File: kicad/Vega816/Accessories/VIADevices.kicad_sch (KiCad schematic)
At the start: 13 parts, among them J102 VIA Port, U125 RC1602A

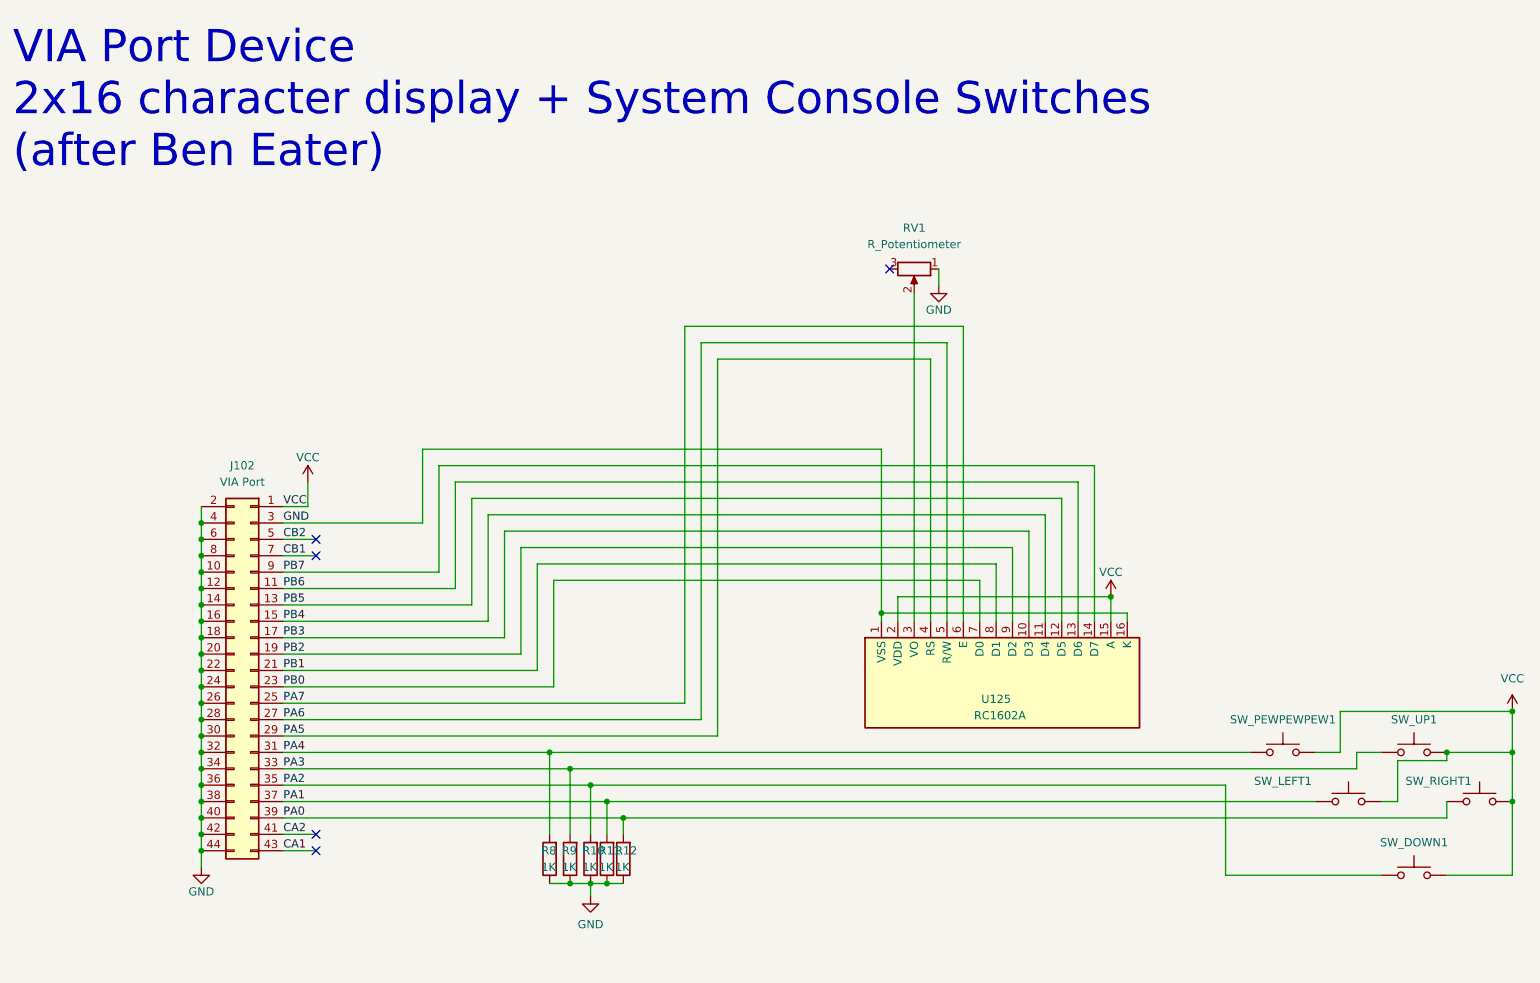
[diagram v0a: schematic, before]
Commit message: via
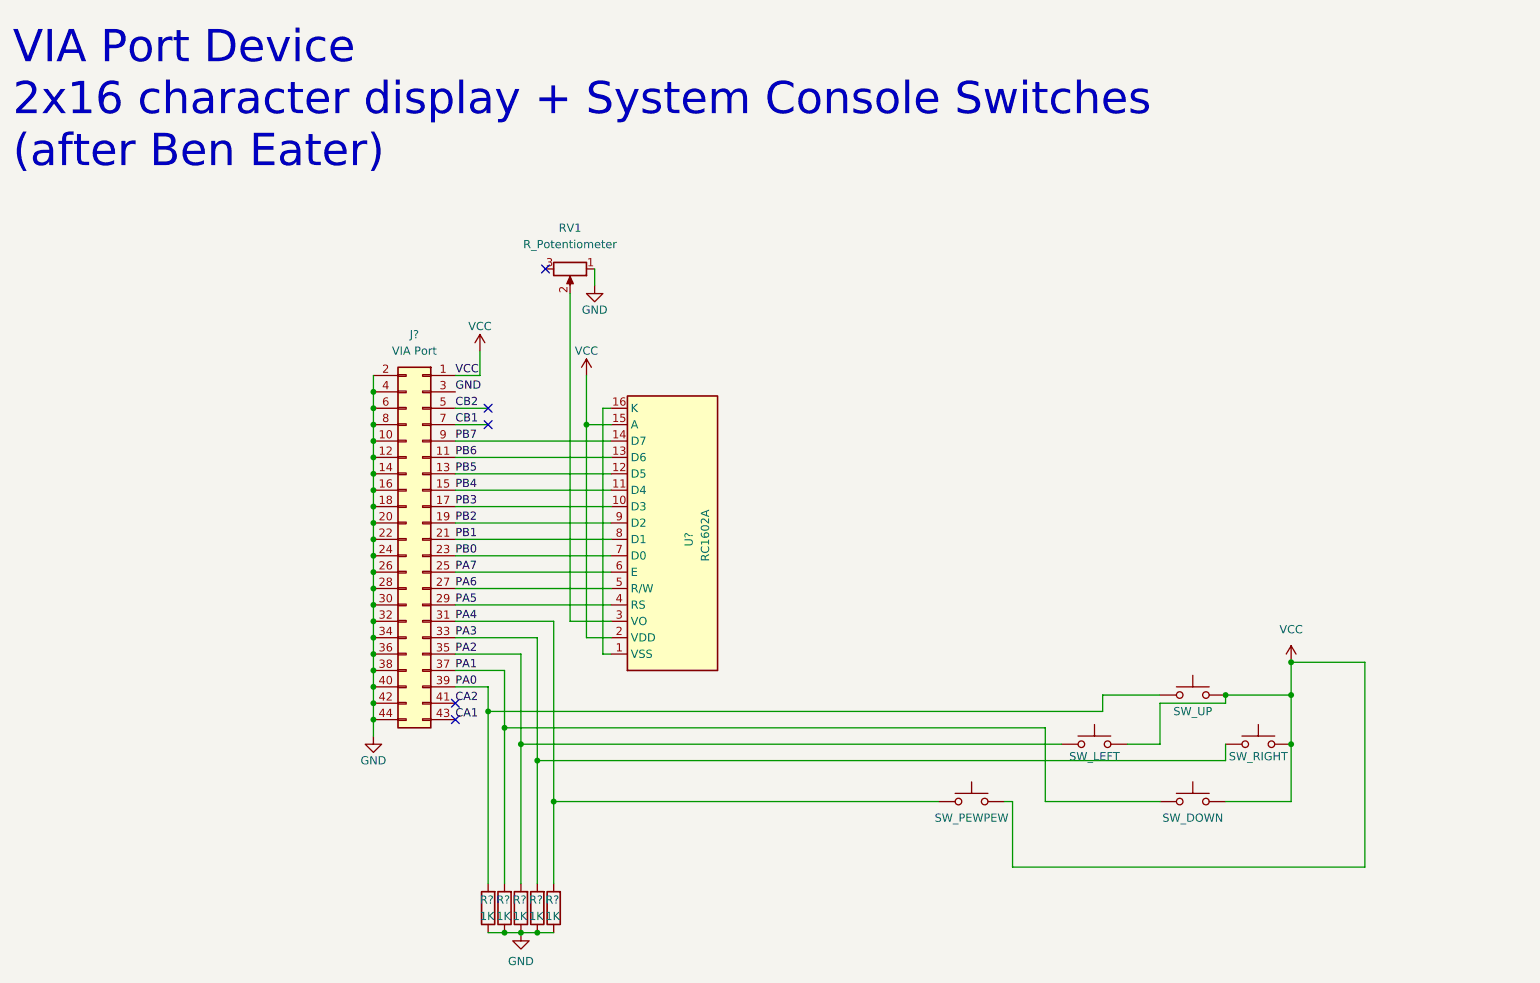
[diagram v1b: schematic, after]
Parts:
- removed J102: VIA Port, symbol Connector_Generic:Conn_02x22_Odd_Even
- removed R10, R11, R12, R8, R9: 1K, symbol Device:R
- removed SW_DOWN1, SW_LEFT1, SW_PEWPEWPEW1, SW_RIGHT1, SW_UP1: SW_Push, symbol Switch:SW_Push
- removed U125: RC1602A, Display:RC1602A, symbol Vega816:RC1602A
- added J?: VIA Port, symbol Connector_Generic:Conn_02x22_Odd_Even
- added R? (x5): 1K, symbol Device:R
- added SW_DOWN, SW_LEFT, SW_PEWPEW, SW_RIGHT, SW_UP: SW_Push, symbol Switch:SW_Push
- added U?: RC1602A, Display:RC1602A, symbol Vega816:RC1602A
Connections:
- net CA1: now also J?.43 (Pin_43)
- net CA2: now also J?.41 (Pin_41)
- net CB1: now also J?.7 (Pin_7)
- net CB2: now also J?.5 (Pin_5)
- net GND: now also J?.10 (Pin_10), J?.12 (Pin_12), J?.14 (Pin_14), J?.16 (Pin_16), J?.18 (Pin_18), J?.2 (Pin_2), J?.20 (Pin_20), J?.22 (Pin_22), J?.24 (Pin_24), J?.26 (Pin_26), J?.28 (Pin_28), J?.3 (Pin_3), J?.30 (Pin_30), J?.32 (Pin_32), J?.34 (Pin_34), J?.36 (Pin_36), J?.38 (Pin_38), J?.4 (Pin_4), J?.40 (Pin_40), J?.42 (Pin_42), J?.44 (Pin_44), J?.6 (Pin_6), J?.8 (Pin_8), R?.1, R?.1, R?.1, R?.1, R?.1
- net PA0: now also J?.39 (Pin_39), R?.2, SW_UP.1
- net PA1: now also J?.37 (Pin_37), R?.2, SW_DOWN.1
- net PA2: now also J?.35 (Pin_35), R?.2, SW_LEFT.1
- net PA3: now also J?.33 (Pin_33), R?.2, SW_RIGHT.1
- net PA4: now also J?.31 (Pin_31), R?.2, SW_PEWPEW.1
- net PA5: now also J?.29 (Pin_29), U?.4 (RS)
- net PA6: now also J?.27 (Pin_27), U?.5 (R/W)
- net PA7: now also J?.25 (Pin_25), U?.6 (E)
- net PB0: now also J?.23 (Pin_23), U?.7 (D0)
- net PB1: now also J?.21 (Pin_21), U?.8 (D1)
- net PB2: now also J?.19 (Pin_19), U?.9 (D2)
- net PB3: now also J?.17 (Pin_17), U?.10 (D3)
- net PB4: now also J?.15 (Pin_15), U?.11 (D4)
- net PB5: now also J?.13 (Pin_13), U?.12 (D5)
- net PB6: now also J?.11 (Pin_11), U?.13 (D6)
- net PB7: now also J?.9 (Pin_9), U?.14 (D7)
- net VCC: now also J?.1 (Pin_1), SW_DOWN.2, SW_LEFT.2, SW_PEWPEW.2, SW_RIGHT.2, SW_UP.2, U?.15 (A), U?.2 (VDD)
- net at RV1.2: now also U?.3 (VO)
- new net: U?.1 (VSS), U?.16 (K)
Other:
- moved on the sheet: RV1

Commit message: dfsg
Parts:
- removed J?: VIA Port, symbol Connector_Generic:Conn_02x22_Odd_Even
- removed R? (x5): 1K, symbol Device:R
- removed RV1: R_Potentiometer, symbol Device:R_Potentiometer
- removed SW_DOWN, SW_LEFT, SW_PEWPEW, SW_RIGHT, SW_UP: SW_Push, symbol Switch:SW_Push
- removed U?: RC1602A, Display:RC1602A, symbol Vega816:RC1602A
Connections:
- no-connect marks 5 -> 0
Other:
- note removed: "VIA Port Device 2x16 character display + System Console Switches (after Ben Eater)"
